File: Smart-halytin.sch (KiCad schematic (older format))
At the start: 17 parts, among them SW1 SW_Push, U1 LPC1113FBD48-302, U3 NHD-C0220BIZ, U4 AMG8854, U5 ESP-07, U6 RN4871, U8 EKMC1607111

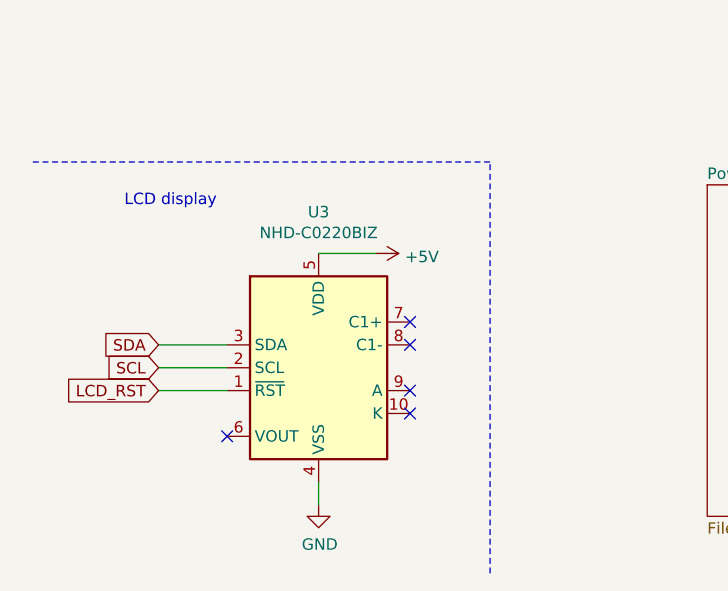
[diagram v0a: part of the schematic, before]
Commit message: lcd connector
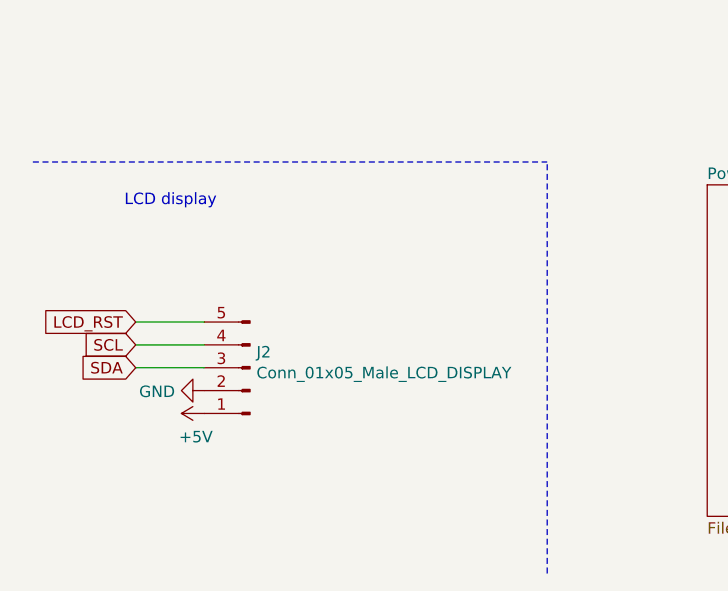
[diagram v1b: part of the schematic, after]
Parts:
- removed U3: NHD-C0220BIZ, Display:NHD-C0220BiZ, symbol Display_Character:NHD-C0220BIZ
- added J2: Conn_01x05_Male_LCD_DISPLAY, Connector_JST:JST_VH_B5P-VH-FB-B_1x05_P3.96mm_Vertical, symbol Connector:Conn_01x05_Male
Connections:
- net +5V: now also J2.1 (Pin_1)
- net GND: now also J2.2 (Pin_2)
- net LCD_RST: now also J2.5 (Pin_5)
- net SCL: now also J2.4 (Pin_4)
- net SDA: now also J2.3 (Pin_3)
- no-connect marks 51 -> 46
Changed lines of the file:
@@
 Wire Wire Line
 	2350 4000 2150 4000
-Text GLabel 1000 6800 0    50   Input ~ 0
+Text GLabel 900  6900 0    50   Input ~ 0
 SDA
-Text GLabel 1000 6900 0    50   Input ~ 0
+Text GLabel 900  6800 0    50   Input ~ 0
 SCL
 $Comp
 L power:GND #PWR0108
 U 1 1 6079DB42
-P 1700 7500
-F 0 "#PWR0108" H 1700 7250 50  0001 C CNN
-F 1 "GND" H 1705 7327 50  0000 C CNN
-F 2 "" H 1700 7500 50  0001 C CNN
-F 3 "" H 1700 7500 50  0001 C CNN
-	1    1700 7500
-	1    0    0    -1
-$EndComp
-Wire Wire Line
-	1700 7400 1700 7500
-Wire Wire Line
-	1000 6800 1300 6800
-Wire Wire Line
-	1000 6900 1300 6900
-NoConn ~ 2100 6700
-NoConn ~ 2100 6800
-NoConn ~ 1300 7200
-Text GLabel 1000 7000 0    50   Input ~ 0
+P 1200 7000
+F 0 "#PWR0108" H 1200 6750 50  0001 C CNN
+F 1 "GND" V 1205 6872 50  0000 R CNN
+F 2 "" H 1200 7000 50  0001 C CNN
+F 3 "" H 1200 7000 50  0001 C CNN
+	1    1200 7000
+	0    1    1    0
+$EndComp
+Wire Wire Line
+	900  6900 1200 6900
+Wire Wire Line
+	900  6800 1200 6800
+Text GLabel 900  6700 0    50   Input ~ 0
 LCD_RST
 Wire Wire Line
-	1000 7000 1300 7000
-NoConn ~ 2100 7000
-NoConn ~ 2100 7100
+	900  6700 1200 6700
 $Comp
 L power:+5V #PWR0109
 U 1 1 607A47EB
-P 1950 6400
-F 0 "#PWR0109" H 1950 6250 50  0001 C CNN
-F 1 "+5V" V 1965 6528 50  0000 L CNN
-F 2 "" H 1950 6400 50  0001 C CNN
-F 3 "" H 1950 6400 50  0001 C CNN
-	1    1950 6400
-	0    1    1    0
-$EndComp
-$Comp
-L Display_Character:NHD-C0220BIZ U3
-U 1 1 6075EF70
-P 1700 6900
-F 0 "U3" H 1700 7581 50  0000 C CNN
-F 1 "NHD-C0220BIZ" H 1700 7490 50  0000 C CNN
-F 2 "Display:NHD-C0220BiZ" H 1700 6300 50  0001 C CNN
-F 3 "http://www.newhavendisplay.com/specs/NHD-C0220BiZ-FSW-FBW-3V3M.pdf" H 1400 7500 50  0001 C CNN
-	1    1700 6900
-	1    0    0    -1
-$EndComp
-Wire Wire Line
-	1700 6400 1950 6400
-Wire Notes Line
-	2450 7800 2450 6000
-Wire Notes Line
-	2450 6000 450  6000
+P 1200 7100
+F 0 "#PWR0109" H 1200 6950 50  0001 C CNN
+F 1 "+5V" V 1097 7137 50  0000 C CNN
+F 2 "" H 1200 7100 50  0001 C CNN
+F 3 "" H 1200 7100 50  0001 C CNN
+	1    1200 7100
+	0    -1   -1   0
+$EndComp
+Wire Notes Line
+	2700 7800 2700 6000
 NoConn ~ 11100 5350
 NoConn ~ 11100 5450
@@
 Wire Wire Line
 	9700 2050 10050 2050
+$Comp
+L Connector:Conn_01x05_Male J2
+U 1 1 608C03CF
+P 1400 6900
+F 0 "J2" H 1372 6832 50  0000 R CNN
+F 1 "Conn_01x05_Male_LCD_DISPLAY" H 1372 6923 50  0000 R CNN
+F 2 "Connector_JST:JST_VH_B5P-VH-FB-B_1x05_P3.96mm_Vertical" H 1400 6900 50  0001 C CNN
+F 3 "~" H 1400 6900 50  0001 C CNN
+	1    1400 6900
+	-1   0    0    1
+$EndComp
+Wire Notes Line
+	450  6000 2700 6000
 $EndSCHEMATC
